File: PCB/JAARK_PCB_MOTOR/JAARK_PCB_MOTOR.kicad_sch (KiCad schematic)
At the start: 32 parts, among them IC1 TPS564242DRLR, IC10 DRV8231DDAR, IC9 DRV8231DDAR, J1 Battery Terminal, J2 Morpho_x2_SSW-119-01-T-D, J3 HC-05, Q1 SSM3J334RLF, Q3 BC237B, U1 4A

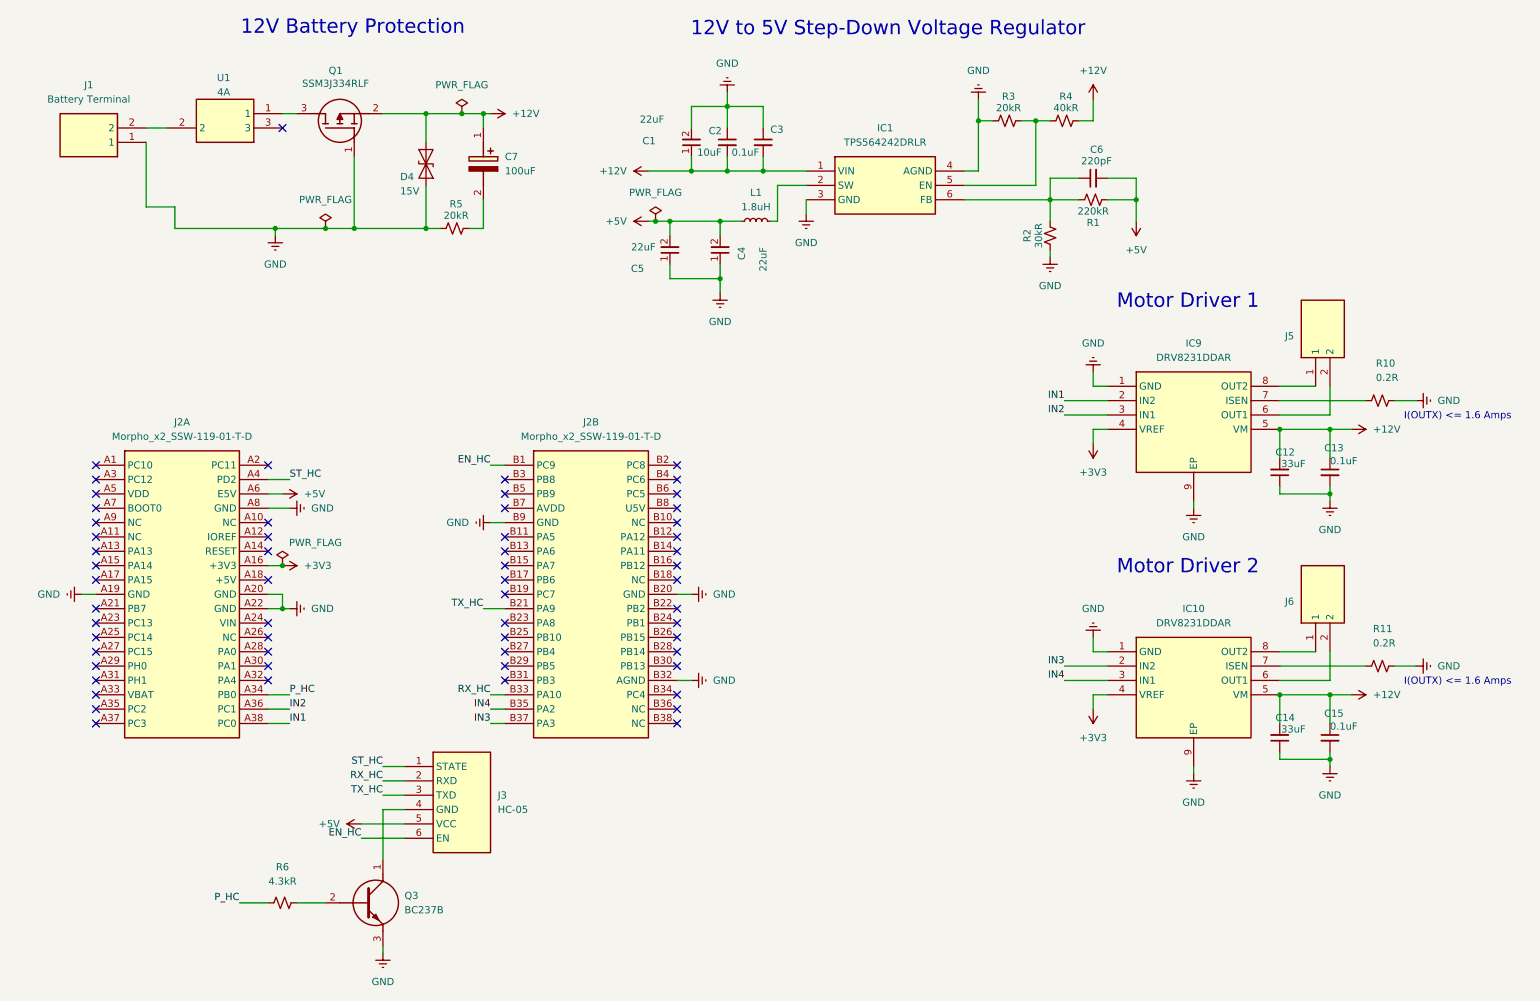
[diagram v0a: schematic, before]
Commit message: Motor PCB finished?
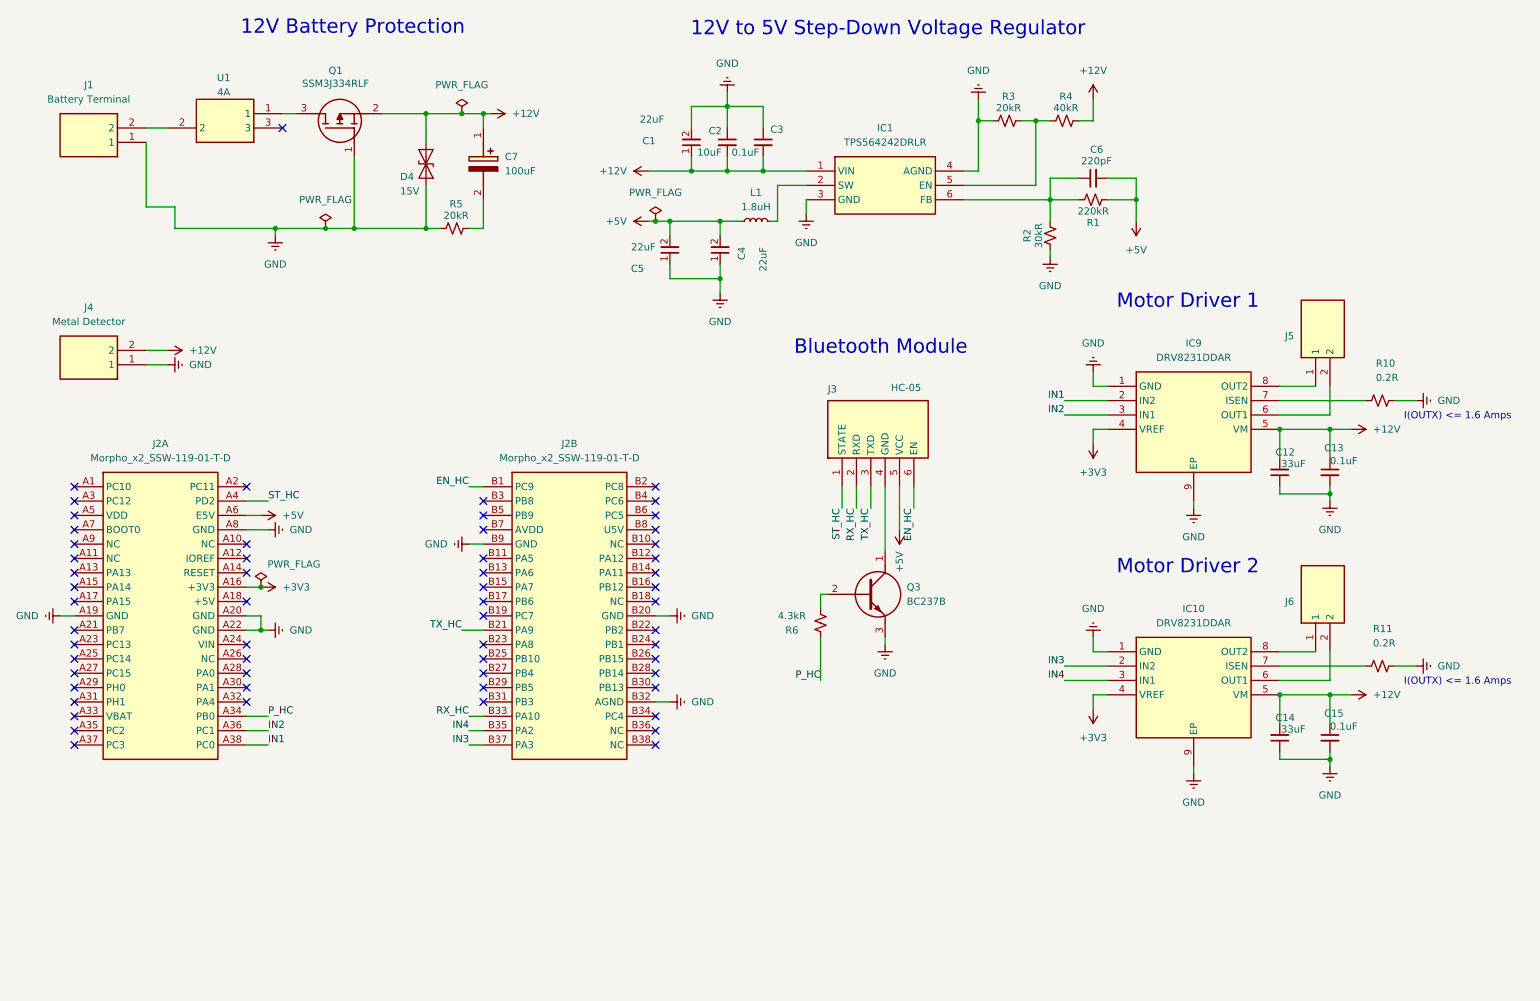
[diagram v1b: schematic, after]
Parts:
- added J4: Metal Detector, JAARK_lib:1984617, symbol SSys_Parts:1984617
- R2: footprint JAARK_lib:RESC2012X60N -> JAARK_lib:RESC2012X65N; Height 0.6 -> 0.65; Manufacturer_Name KEMET -> TE Connectivity; Manufacturer_Part_Number RC0805FR-0730K1L -> CRG0805F30K; Mouser Part Number 603-RC0805FR-0730K1L -> 279-CRG0805F30K; Mouser Price/Stock https://www.mouser.com/Search/Refine.aspx?Keyword=603-RC080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 -> https://www.mouser.co.uk/ProductDetail/TE-Connectivity-Hols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
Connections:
- net +12V: now also J4.2
- net GND: now also J4.1
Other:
- note added: "Bluetooth Module"
- moved on the sheet: J2A, J2B, J3, Q3, R6
